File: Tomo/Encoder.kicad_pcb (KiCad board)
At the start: 2 copper layers, 24 x 24 mm, 8 parts, among them J1 CONN_01X04, J201 CONN_01X01, J202 CONN_01X01, U000 QRE1113, U1 KwanSystems, U100 QRE1113

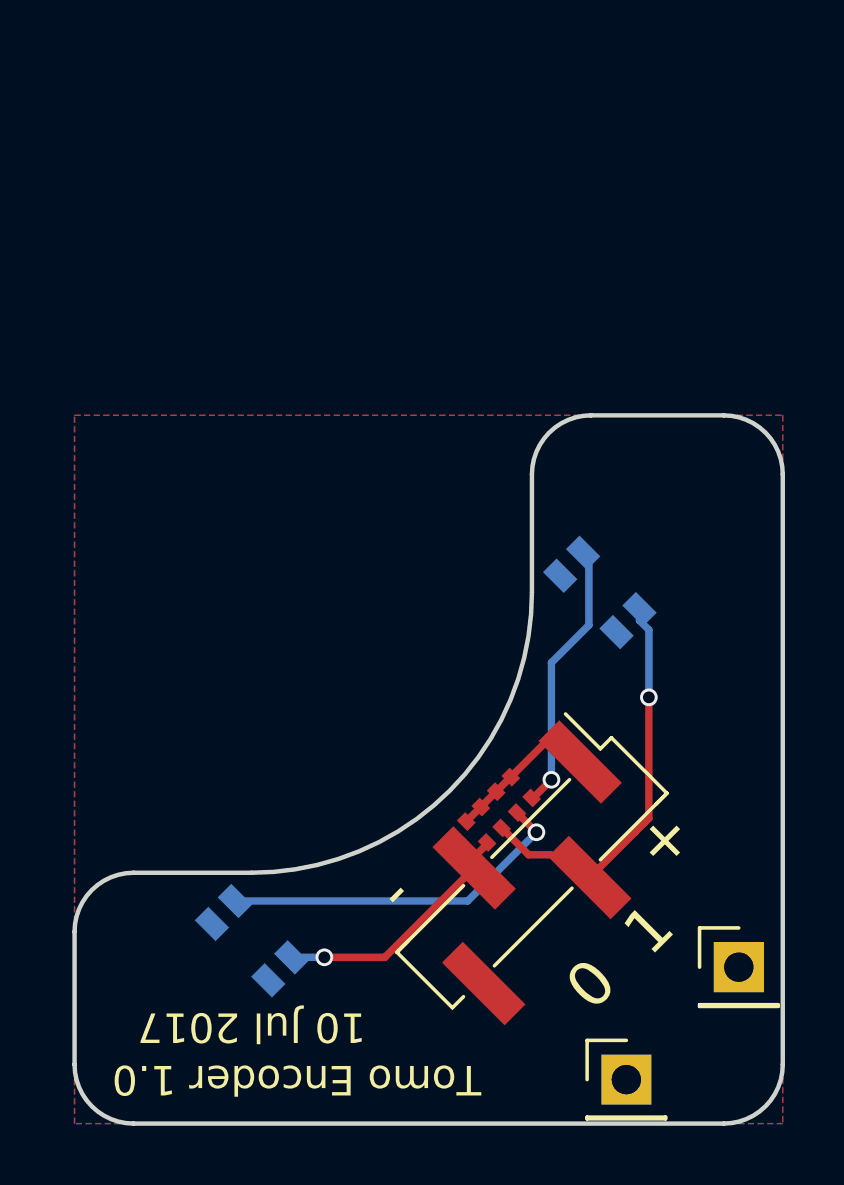
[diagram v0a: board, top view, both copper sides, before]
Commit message: Files as ordered
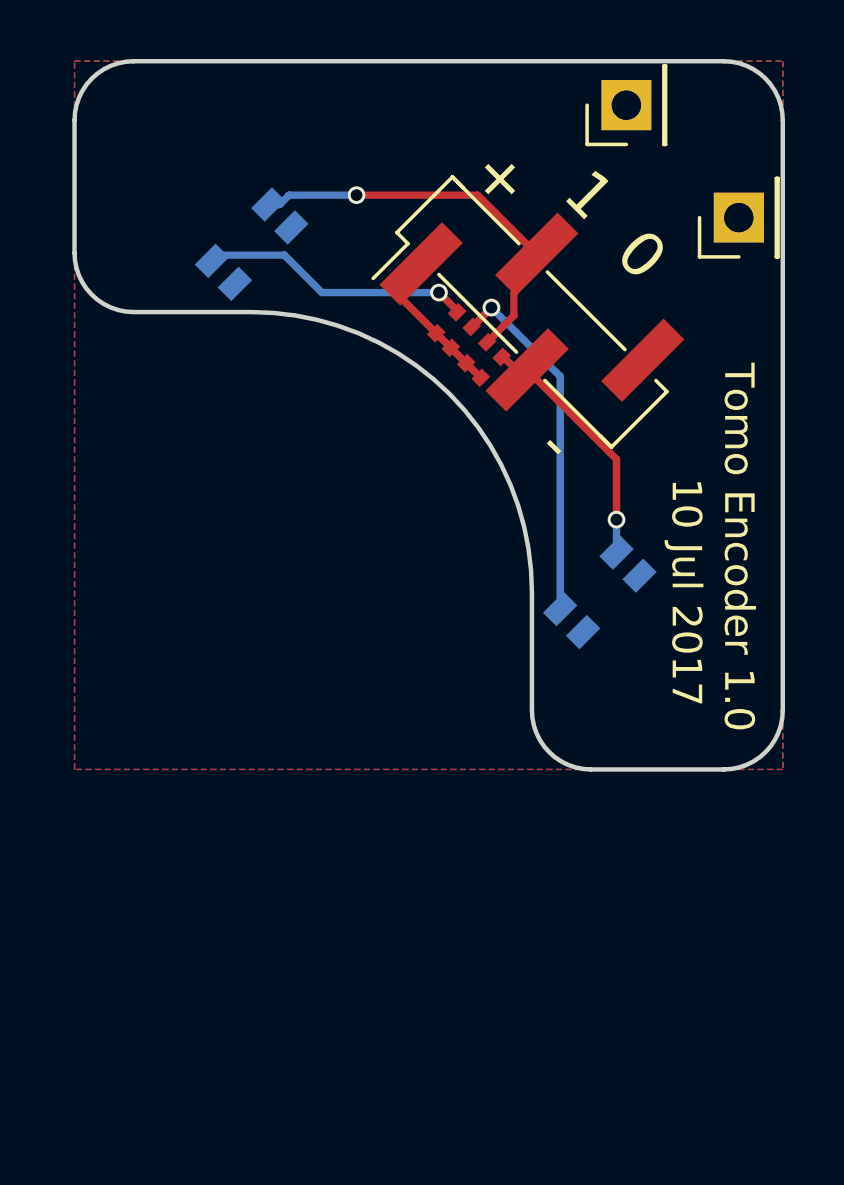
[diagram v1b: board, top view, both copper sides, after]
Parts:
- moved J201 29.5 mm to (116.5, 87.3), turned to 90 degrees
- moved J202 29.5 mm to (112.7, 83.5), turned to 90 degrees
- moved U1 19.7 mm to (98.2, 86.0), turned to 0 degrees
- moved J1 19.0 mm to (109.5, 90.5), turned to 45 degrees
- moved U000 16.7 mm to (111.8, 100.0), turned to 225 degrees
- moved U100 16.7 mm to (100.0, 88.2), turned to 225 degrees
- moved R2 15.9 mm to (106.9, 91.1), turned to 45 degrees
- moved R1 15.7 mm to (107.9, 92.1), turned to 45 degrees
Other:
- outline, holes or cut-outs redrawn
